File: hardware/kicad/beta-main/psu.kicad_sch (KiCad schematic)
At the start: 0 parts

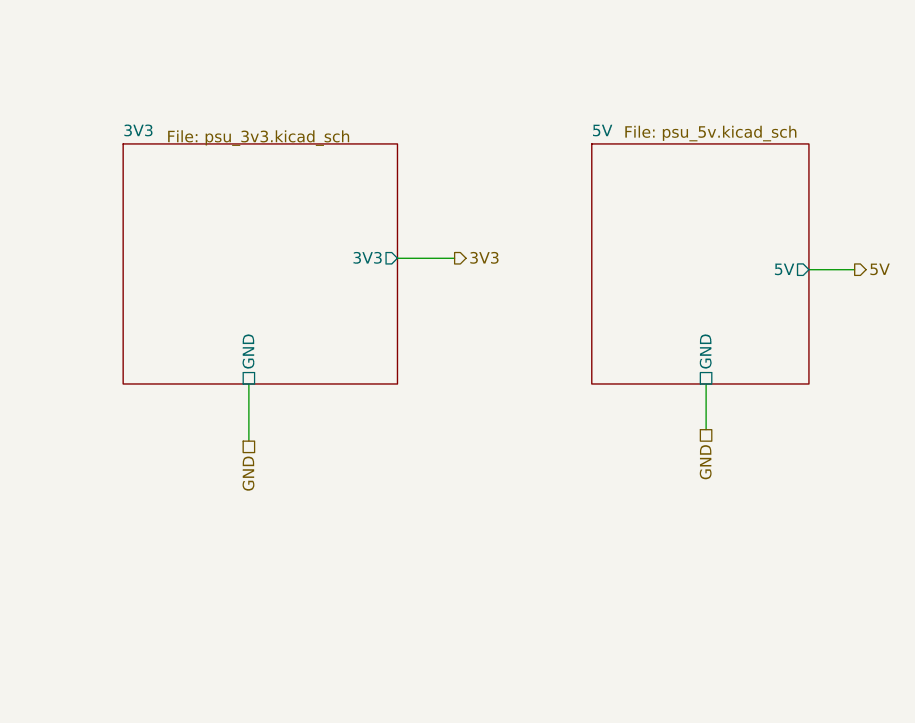
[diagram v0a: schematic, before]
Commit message: tweaks and added servo controller
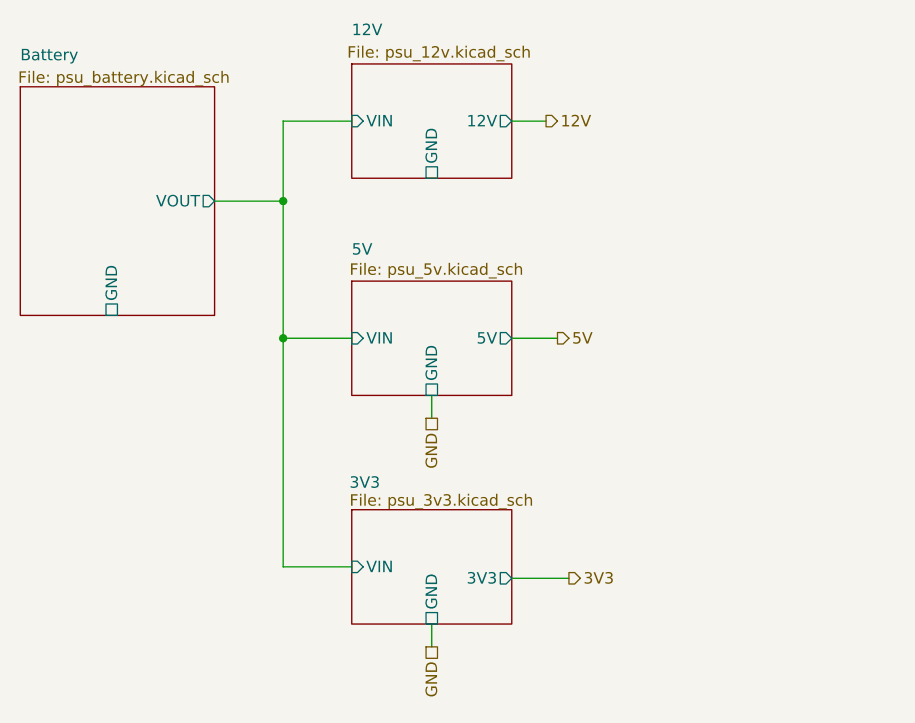
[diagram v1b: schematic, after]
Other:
- added sheet 12V (psu_12v.kicad_sch)
- added sheet Battery (psu_battery.kicad_sch)
- sheet 3V3 ports: added VIN; removed none
- sheet 5V ports: added VIN; removed none
